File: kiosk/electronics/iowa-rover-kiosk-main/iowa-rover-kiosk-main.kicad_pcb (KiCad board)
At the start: 2 copper layers, 76.8 x 79.9 mm, 18 parts, among them J2 Barrel_Jack, J3 Conn_02x06_Odd_Even, J4 Conn_01x04, J5 Conn_02x08_Top_Bottom, J6 Conn_01x08, J7 Conn_01x03, U1 Adafruit_RFM69HCW_Breakout, U2 I50115, U3 ATtiny84-20P

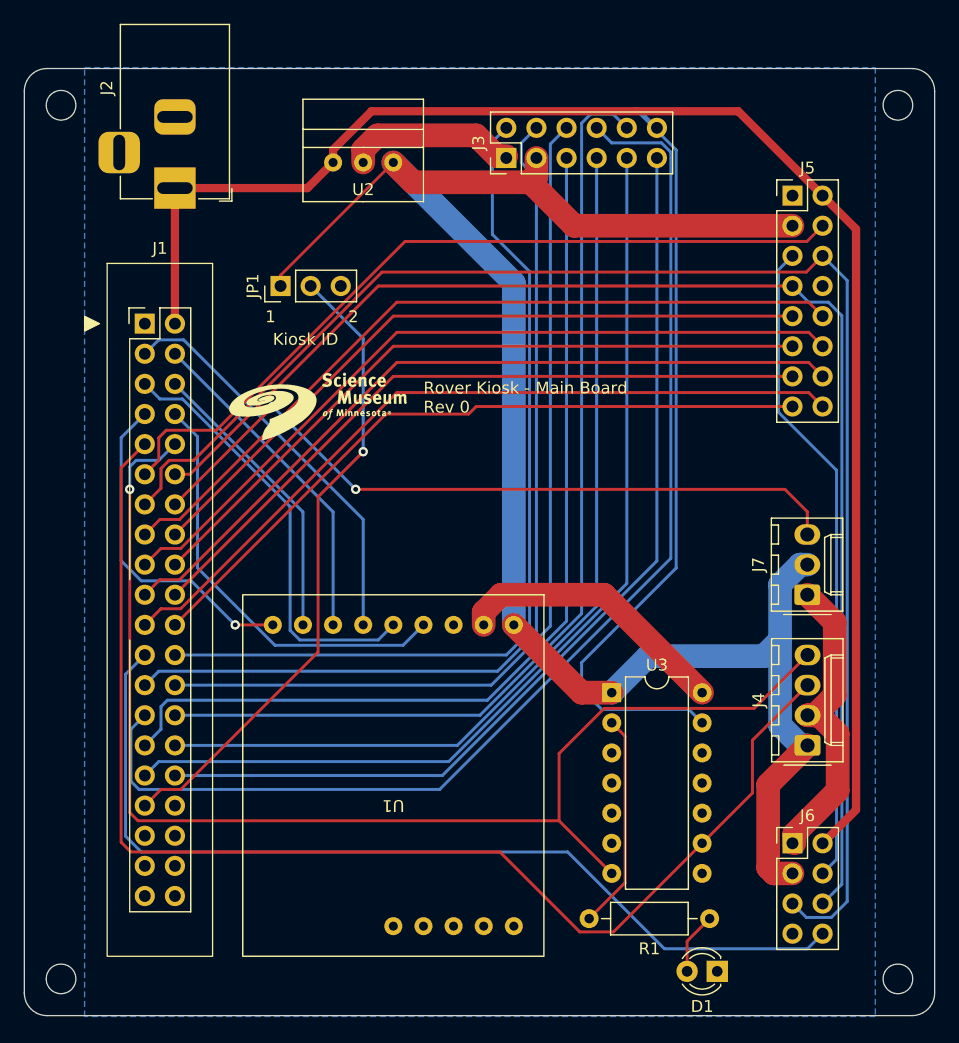
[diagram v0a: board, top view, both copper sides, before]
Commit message: update
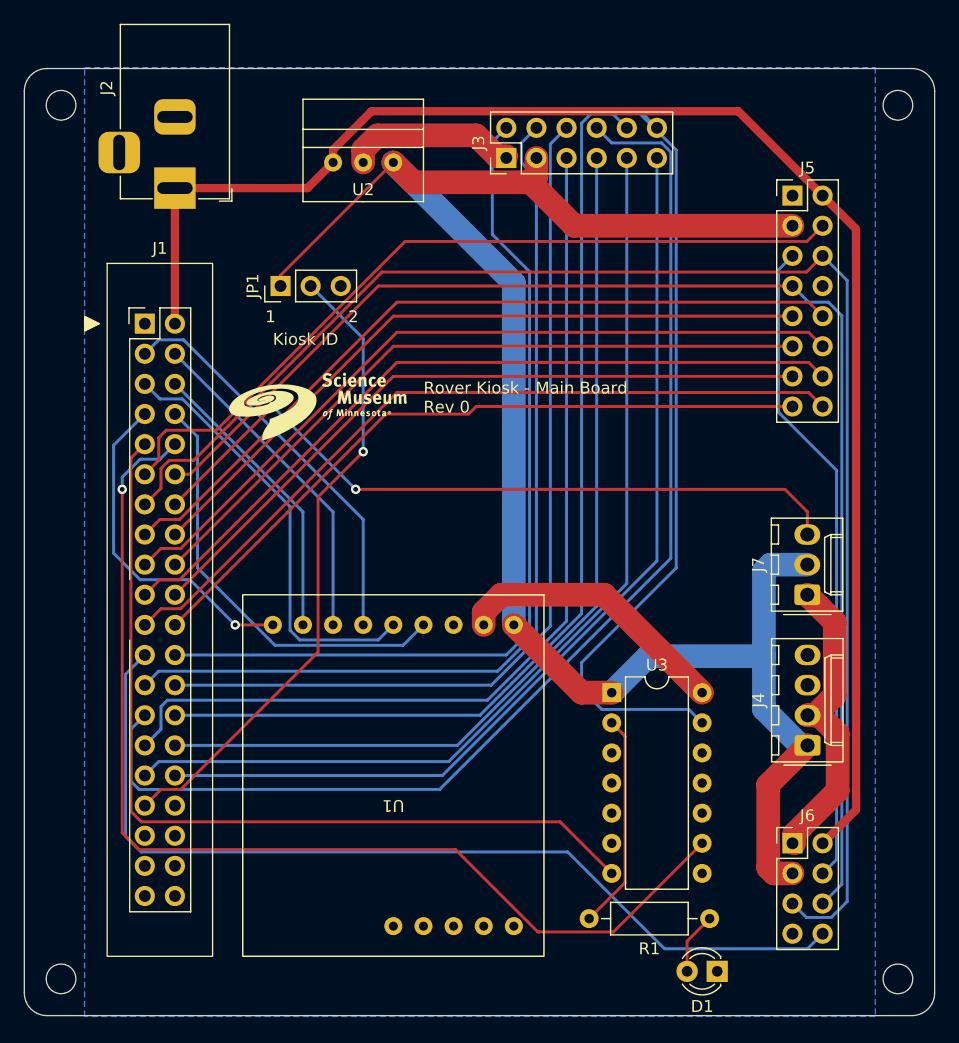
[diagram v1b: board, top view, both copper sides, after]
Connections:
- U3 pad 7: /SCL -> /SDA
- U3 pad 9: /SDA -> /SCL
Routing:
- net /SDA: track 106.6 -> 74.2 mm
- net /SCL: track 106.6 -> 91.0 mm
- net +5V: track 154.1 -> 154.8 mm
- net Net-(J1-D45_RST): track 28.1 -> 28.7 mm
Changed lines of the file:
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@@
       (net 57 "unconnected-(U3-PA7-Pad6)") (pinfunction "PA7") (pintype "bidirectional+no_connect"))
     (pad "7" thru_hole oval (at 0 15.24) (size 1.6 1.6) (drill 0.8) (layers "*.Cu" "*.Mask")
-      (net 11 "/SCL") (pinfunction "PA6") (pintype "bidirectional"))
+      (net 10 "/SDA") (pinfunction "PA6") (pintype "bidirectional"))
     (pad "8" thru_hole oval (at 7.62 15.24) (size 1.6 1.6) (drill 0.8) (layers "*.Cu" "*.Mask")
       (net 58 "unconnected-(U3-PA5-Pad8)") (pinfunction "PA5") (pintype "bidirectional+no_connect"))
     (pad "9" thru_hole oval (at 7.62 12.7) (size 1.6 1.6) (drill 0.8) (layers "*.Cu" "*.Mask")
-      (net 10 "/SDA") (pinfunction "PA4") (pintype "bidirectional"))
+      (net 11 "/SCL") (pinfunction "PA4") (pintype "bidirectional"))
     (pad "10" thru_hole oval (at 7.62 10.16) (size 1.6 1.6) (drill 0.8) (layers "*.Cu" "*.Mask")
       (net 59 "unconnected-(U3-PA3-Pad10)") (pinfunction "PA3") (pintype "bidirectional+no_connect"))
@@
   (segment (start 58.42 93.98) (end 55.335 93.98) (width 0.25) (layer "F.Cu") (net 8))
   (via (at 55.245 93.98) (size 0.8) (drill 0.4) (layers "F.Cu" "B.Cu") (net 8))
-  (segment (start 55.245 93.98) (end 51.53 90.265) (width 0.25) (layer "B.Cu") (net 8))
-  (segment (start 47.328299 90.265) (end 45.63 88.566701) (width 0.25) (layer "B.Cu") (net 8))
-  (segment (start 45.63 78.195) (end 47.625 76.2) (width 0.25) (layer "B.Cu") (net 8))
-  (segment (start 45.63 88.566701) (end 45.63 78.195) (width 0.25) (layer "B.Cu") (net 8))
-  (segment (start 51.53 90.265) (end 47.328299 90.265) (width 0.25) (layer "B.Cu") (net 8))
+  (segment (start 47.233299 90.17) (end 51.435 90.17) (width 0.25) (layer "B.Cu") (net 8))
+  (segment (start 51.435 90.17) (end 55.245 93.98) (width 0.25) (layer "B.Cu") (net 8))
+  (segment (start 47.625 76.2) (end 44.995 78.83) (width 0.25) (layer "B.Cu") (net 8))
+  (segment (start 44.995 78.83) (end 44.995 87.931701) (width 0.25) (layer "B.Cu") (net 8))
+  (segment (start 44.995 87.931701) (end 47.233299 90.17) (width 0.25) (layer "B.Cu") (net 8))
   (segment (start 69.4 95.7) (end 58.602749 95.7) (width 0.25) (layer "B.Cu") (net 9))
   (segment (start 71.12 93.98) (end 69.4 95.7) (width 0.25) (layer "B.Cu") (net 9))
@@
   (segment (start 58.602749 95.7) (end 52.069302 89.166553) (width 0.25) (layer "B.Cu") (net 9))
   (segment (start 52.069302 89.166553) (end 52.069302 78.104302) (width 0.25) (layer "B.Cu") (net 9))
-  (segment (start 45.63 112.305) (end 46.45 113.125) (width 0.25) (layer "F.Cu") (net 10))
-  (segment (start 98.86 108.15) (end 98.86 103.705) (width 0.25) (layer "F.Cu") (net 10))
-  (segment (start 84.31 119.87) (end 87.14 119.87) (width 0.25) (layer "F.Cu") (net 10))
-  (segment (start 47.625 78.74) (end 45.63 80.735) (width 0.25) (layer "F.Cu") (net 10))
-  (segment (start 98.86 103.705) (end 103.505 99.06) (width 0.25) (layer "F.Cu") (net 10))
-  (segment (start 45.63 80.735) (end 45.63 112.305) (width 0.25) (layer "F.Cu") (net 10))
-  (segment (start 46.45 113.125) (end 77.565 113.125) (width 0.25) (layer "F.Cu") (net 10))
-  (segment (start 94.615 112.395) (end 98.86 108.15) (width 0.25) (layer "F.Cu") (net 10))
-  (segment (start 77.565 113.125) (end 84.31 119.87) (width 0.25) (layer "F.Cu") (net 10))
-  (segment (start 87.14 119.87) (end 94.615 112.395) (width 0.25) (layer "F.Cu") (net 10))
-  (segment (start 82.55 110.49) (end 86.995 114.935) (width 0.25) (layer "F.Cu") (net 11))
-  (segment (start 86.36 101.02) (end 99.005 101.02) (width 0.25) (layer "F.Cu") (net 11))
-  (segment (start 82.55 110.49) (end 82.55 104.83) (width 0.25) (layer "F.Cu") (net 11))
-  (segment (start 46.355 82.55) (end 46.355 109.801701) (width 0.25) (layer "F.Cu") (net 11))
-  (segment (start 99.005 101.02) (end 103.505 96.52) (width 0.25) (layer "F.Cu") (net 11))
-  (segment (start 46.355 109.801701) (end 47.043299 110.49) (width 0.25) (layer "F.Cu") (net 11))
-  (segment (start 82.55 104.83) (end 86.36 101.02) (width 0.25) (layer "F.Cu") (net 11))
-  (segment (start 47.043299 110.49) (end 82.55 110.49) (width 0.25) (layer "F.Cu") (net 11))
-  (via (at 46.355 82.55) (size 0.8) (drill 0.4) (layers "F.Cu" "B.Cu") (net 11))
-  (segment (start 48.8 80.105) (end 50.165 78.74) (width 0.25) (layer "B.Cu") (net 11))
-  (segment (start 46.355 80.645) (end 46.895 80.105) (width 0.25) (layer "B.Cu") (net 11))
-  (segment (start 46.355 82.55) (end 46.355 80.645) (width 0.25) (layer "B.Cu") (net 11))
-  (segment (start 46.895 80.105) (end 48.8 80.105) (width 0.25) (layer "B.Cu") (net 11))
+  (segment (start 82.645 110.585) (end 86.995 114.935) (width 0.25) (layer "F.Cu") (net 10))
+  (segment (start 47.625 78.74) (end 46.45 79.915) (width 0.25) (layer "F.Cu") (net 10))
+  (segment (start 46.45 109.706701) (end 47.328299 110.585) (width 0.25) (layer "F.Cu") (net 10))
+  (segment (start 46.45 79.915) (end 46.45 109.706701) (width 0.25) (layer "F.Cu") (net 10))
+  (segment (start 47.328299 110.585) (end 82.645 110.585) (width 0.25) (layer "F.Cu") (net 10))
+  (segment (start 73.832251 112.935) (end 47.138299 112.935) (width 0.25) (layer "F.Cu") (net 11))
+  (segment (start 87.14 119.87) (end 80.767251 119.87) (width 0.25) (layer "F.Cu") (net 11))
+  (segment (start 94.615 112.395) (end 87.14 119.87) (width 0.25) (layer "F.Cu") (net 11))
+  (segment (start 80.767251 119.87) (end 73.832251 112.935) (width 0.25) (layer "F.Cu") (net 11))
+  (segment (start 45.72 111.516701) (end 45.72 82.55) (width 0.25) (layer "F.Cu") (net 11))
+  (segment (start 47.138299 112.935) (end 45.72 111.516701) (width 0.25) (layer "F.Cu") (net 11))
+  (via (at 45.72 82.55) (size 0.8) (drill 0.4) (layers "F.Cu" "B.Cu") (net 11))
+  (segment (start 47.233299 80.01) (end 48.895 80.01) (width 0.25) (layer "B.Cu") (net 11))
+  (segment (start 45.72 81.523299) (end 47.233299 80.01) (width 0.25) (layer "B.Cu") (net 11))
+  (segment (start 45.72 82.55) (end 45.72 81.523299) (width 0.25) (layer "B.Cu") (net 11))
+  (segment (start 48.895 80.01) (end 50.165 78.74) (width 0.25) (layer "B.Cu") (net 11))
   (segment (start 49.435 77.565) (end 48.8 78.2) (width 0.25) (layer "F.Cu") (net 12))
   (segment (start 48.8 78.2) (end 48.8 80.105) (width 0.25) (layer "F.Cu") (net 12))
@@
   (segment (start 84.455 99.695) (end 78.74 93.98) (width 2) (layer "F.Cu") (net 42))
   (segment (start 100.185 114.445) (end 100.675 114.935) (width 2) (layer "F.Cu") (net 42))
-  (segment (start 101.19 102.437422) (end 102.892578 104.14) (width 2) (layer "B.Cu") (net 42))
-  (segment (start 102.872578 88.9) (end 101.19 90.582578) (width 2) (layer "B.Cu") (net 42))
+  (segment (start 102.892578 104.14) (end 99.825 101.072422) (width 2) (layer "B.Cu") (net 42))
   (segment (start 86.995 99.695) (end 90.075 96.615) (width 2) (layer "B.Cu") (net 42))
-  (segment (start 99.825 96.615) (end 101.19 95.25) (width 2) (layer "B.Cu") (net 42))
+  (segment (start 99.825 101.072422) (end 99.825 96.615) (width 2) (layer "B.Cu") (net 42))
+  (segment (start 99.825 89.465) (end 100.39 88.9) (width 2) (layer "B.Cu") (net 42))
   (segment (start 68.58 54.991) (end 78.74 65.151) (width 2) (layer "B.Cu") (net 42))
   (segment (start 90.075 96.615) (end 99.825 96.615) (width 2) (layer "B.Cu") (net 42))
-  (segment (start 102.892578 104.14) (end 103.505 104.14) (width 2) (layer "B.Cu") (net 42))
-  (segment (start 101.19 95.25) (end 101.19 102.437422) (width 2) (layer "B.Cu") (net 42))
+  (segment (start 99.825 96.615) (end 99.825 89.465) (width 2) (layer "B.Cu") (net 42))
+  (segment (start 100.39 88.9) (end 103.485 88.9) (width 2) (layer "B.Cu") (net 42))
   (segment (start 78.74 65.151) (end 78.74 93.98) (width 2) (layer "B.Cu") (net 42))
-  (segment (start 103.485 88.9) (end 102.872578 88.9) (width 2) (layer "B.Cu") (net 42))
-  (segment (start 101.19 90.582578) (end 101.19 95.25) (width 2) (layer "B.Cu") (net 42))
+  (segment (start 103.505 104.14) (end 102.892578 104.14) (width 2) (layer "B.Cu") (net 42))
   (segment (start 92.43 89.18) (end 84.455 97.155) (width 0.25) (layer "B.Cu") (net 43))
   (segment (start 84.455 99.405) (end 86.16 101.11) (width 0.25) (layer "B.Cu") (net 43))
